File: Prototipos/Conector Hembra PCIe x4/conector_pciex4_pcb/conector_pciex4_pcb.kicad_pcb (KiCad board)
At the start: 2 copper layers, 16.4 x 39.7 mm, 33 parts, among them J1 10018783-10211TLF

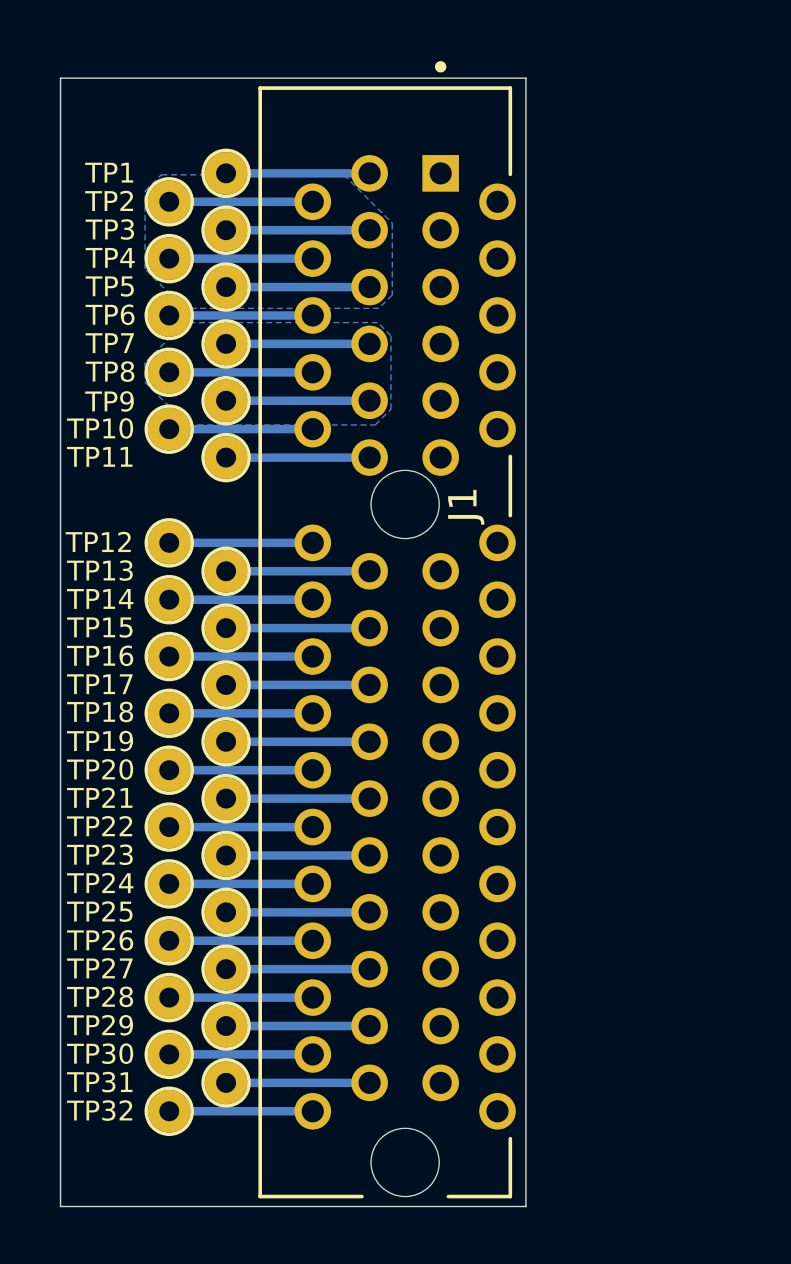
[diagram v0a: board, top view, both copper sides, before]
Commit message: Corrección PCB
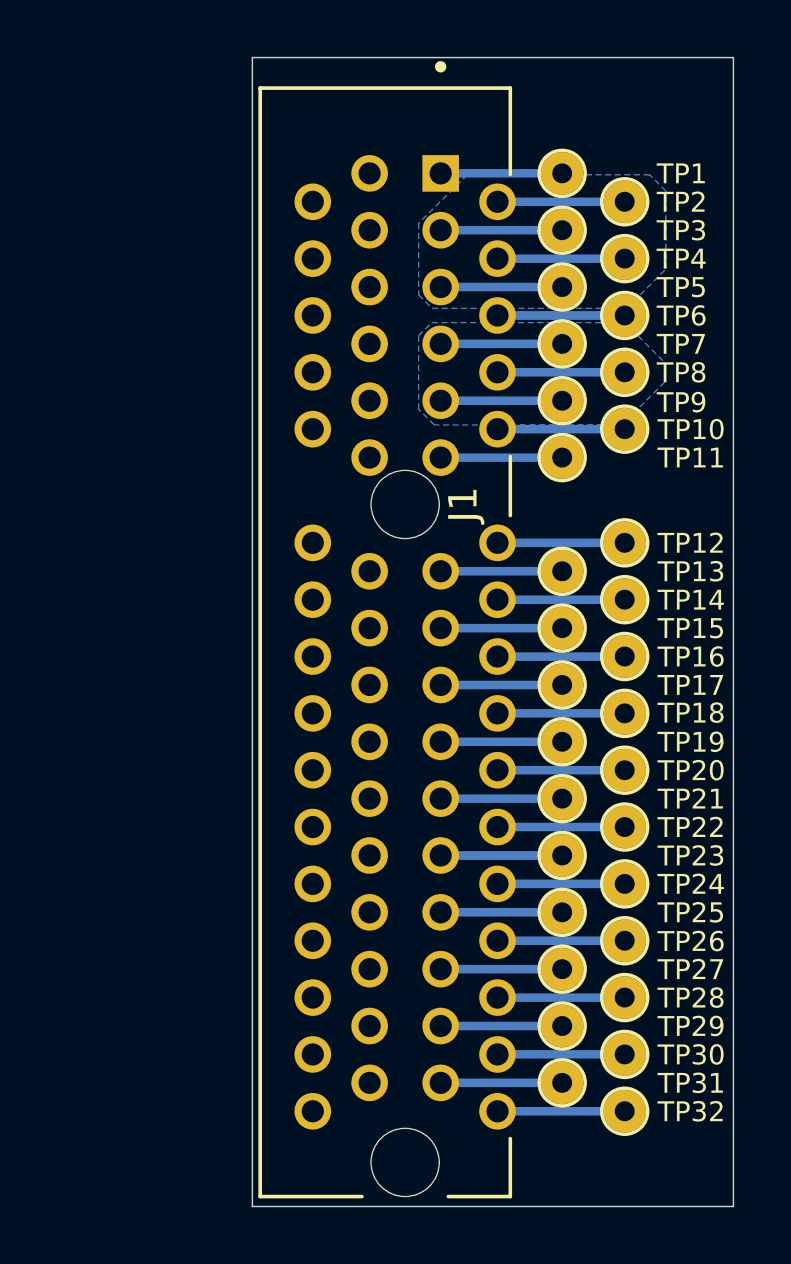
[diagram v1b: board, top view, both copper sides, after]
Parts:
- moved TP10 16.0 mm to (140.4, 73.6)
- moved TP12 16.0 mm to (140.4, 77.6)
- moved TP14 16.0 mm to (140.4, 79.6)
- moved TP16 16.0 mm to (140.4, 81.6)
- moved TP18 16.0 mm to (140.4, 83.6)
- moved TP2 16.0 mm to (140.4, 65.6)
- moved TP20 16.0 mm to (140.4, 85.6)
- moved TP22 16.0 mm to (140.4, 87.6)
- moved TP24 16.0 mm to (140.4, 89.6)
- moved TP26 16.0 mm to (140.4, 91.6)
- moved TP28 16.0 mm to (140.4, 93.6)
- moved TP30 16.0 mm to (140.4, 95.6)
- moved TP32 16.0 mm to (140.4, 97.6)
- moved TP4 16.0 mm to (140.4, 67.6)
- moved TP6 16.0 mm to (140.4, 69.6)
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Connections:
- J1 pad A1: unconnected-(J1-PadA1) -> Net-(J1-PadA1)
- J1 pad A10: unconnected-(J1-PadA10) -> Net-(J1-PadA10)
- J1 pad A11: unconnected-(J1-PadA11) -> Net-(J1-PadA11)
- J1 pad A12: unconnected-(J1-PadA12) -> Net-(J1-PadA12)
- J1 pad A13: unconnected-(J1-PadA13) -> Net-(J1-PadA13)
- J1 pad A14: unconnected-(J1-PadA14) -> Net-(J1-PadA14)
- J1 pad A15: unconnected-(J1-PadA15) -> Net-(J1-PadA15)
- J1 pad A16: unconnected-(J1-PadA16) -> Net-(J1-PadA16)
- J1 pad A17: unconnected-(J1-PadA17) -> Net-(J1-PadA17)
- J1 pad A18: unconnected-(J1-PadA18) -> Net-(J1-PadA18)
- J1 pad A19: unconnected-(J1-PadA19) -> Net-(J1-PadA19)
- J1 pad A2: unconnected-(J1-PadA2) -> Net-(J1-PadA2)
- J1 pad A20: unconnected-(J1-PadA20) -> Net-(J1-PadA20)
- J1 pad A21: unconnected-(J1-PadA21) -> Net-(J1-PadA21)
- J1 pad A22: unconnected-(J1-PadA22) -> Net-(J1-PadA22)
- J1 pad A23: unconnected-(J1-PadA23) -> Net-(J1-PadA23)
- J1 pad A24: unconnected-(J1-PadA24) -> Net-(J1-PadA24)
- J1 pad A25: unconnected-(J1-PadA25) -> Net-(J1-PadA25)
- J1 pad A26: unconnected-(J1-PadA26) -> Net-(J1-PadA26)
- J1 pad A27: unconnected-(J1-PadA27) -> Net-(J1-PadA27)
- J1 pad A28: unconnected-(J1-PadA28) -> Net-(J1-PadA28)
- J1 pad A29: unconnected-(J1-PadA29) -> Net-(J1-PadA29)
- J1 pad A3: unconnected-(J1-PadA3) -> Net-(J1-PadA2)
- J1 pad A30: unconnected-(J1-PadA30) -> Net-(J1-PadA30)
- J1 pad A31: unconnected-(J1-PadA31) -> Net-(J1-PadA31)
- J1 pad A32: unconnected-(J1-PadA32) -> Net-(J1-PadA32)
- J1 pad A4: unconnected-(J1-PadA4) -> Net-(J1-PadA2)
- J1 pad A5: unconnected-(J1-PadA5) -> Net-(J1-PadA2)
- J1 pad A6: unconnected-(J1-PadA6) -> Net-(J1-PadA6)
- J1 pad A7: unconnected-(J1-PadA7) -> Net-(J1-PadA7)
- J1 pad A8: unconnected-(J1-PadA8) -> Net-(J1-PadA7)
- J1 pad A9: unconnected-(J1-PadA9) -> Net-(J1-PadA7)
- J1 pad B1: Net-(J1-PadB1) -> unconnected-(J1-PadB1)
- J1 pad B10: Net-(J1-PadB10) -> unconnected-(J1-PadB10)
- J1 pad B11: Net-(J1-PadB11) -> unconnected-(J1-PadB11)
- J1 pad B12: Net-(J1-PadB12) -> unconnected-(J1-PadB12)
- J1 pad B13: Net-(J1-PadB13) -> unconnected-(J1-PadB13)
- J1 pad B14: Net-(J1-PadB14) -> unconnected-(J1-PadB14)
- J1 pad B15: Net-(J1-PadB15) -> unconnected-(J1-PadB15)
- J1 pad B16: Net-(J1-PadB16) -> unconnected-(J1-PadB16)
- J1 pad B17: Net-(J1-PadB17) -> unconnected-(J1-PadB17)
- J1 pad B18: Net-(J1-PadB18) -> unconnected-(J1-PadB18)
- J1 pad B19: Net-(J1-PadB19) -> unconnected-(J1-PadB19)
- J1 pad B2: Net-(J1-PadB2) -> unconnected-(J1-PadB2)
- J1 pad B20: Net-(J1-PadB20) -> unconnected-(J1-PadB20)
- J1 pad B21: Net-(J1-PadB21) -> unconnected-(J1-PadB21)
- J1 pad B22: Net-(J1-PadB22) -> unconnected-(J1-PadB22)
- J1 pad B23: Net-(J1-PadB23) -> unconnected-(J1-PadB23)
- J1 pad B24: Net-(J1-PadB24) -> unconnected-(J1-PadB24)
- J1 pad B25: Net-(J1-PadB25) -> unconnected-(J1-PadB25)
- J1 pad B26: Net-(J1-PadB26) -> unconnected-(J1-PadB26)
- J1 pad B27: Net-(J1-PadB27) -> unconnected-(J1-PadB27)
- J1 pad B28: Net-(J1-PadB28) -> unconnected-(J1-PadB28)
- J1 pad B29: Net-(J1-PadB29) -> unconnected-(J1-PadB29)
- J1 pad B3: Net-(J1-PadB2) -> unconnected-(J1-PadB3)
- J1 pad B30: Net-(J1-PadB30) -> unconnected-(J1-PadB30)
- J1 pad B31: Net-(J1-PadB31) -> unconnected-(J1-PadB31)
- J1 pad B32: Net-(J1-PadB32) -> unconnected-(J1-PadB32)
- J1 pad B4: Net-(J1-PadB2) -> unconnected-(J1-PadB4)
- J1 pad B5: Net-(J1-PadB2) -> unconnected-(J1-PadB5)
- J1 pad B6: Net-(J1-PadB6) -> unconnected-(J1-PadB6)
- J1 pad B7: Net-(J1-PadB7) -> unconnected-(J1-PadB7)
- J1 pad B8: Net-(J1-PadB7) -> unconnected-(J1-PadB8)
- J1 pad B9: Net-(J1-PadB7) -> unconnected-(J1-PadB9)
- TP1 pad 1: Net-(J1-PadB1) -> Net-(J1-PadA1)
- TP10 pad 1: Net-(J1-PadB10) -> Net-(J1-PadA10)
- TP11 pad 1: Net-(J1-PadB11) -> Net-(J1-PadA11)
- TP12 pad 1: Net-(J1-PadB12) -> Net-(J1-PadA12)
- TP13 pad 1: Net-(J1-PadB13) -> Net-(J1-PadA13)
- TP14 pad 1: Net-(J1-PadB14) -> Net-(J1-PadA14)
- TP15 pad 1: Net-(J1-PadB15) -> Net-(J1-PadA15)
- TP16 pad 1: Net-(J1-PadB16) -> Net-(J1-PadA16)
- TP17 pad 1: Net-(J1-PadB17) -> Net-(J1-PadA17)
- TP18 pad 1: Net-(J1-PadB18) -> Net-(J1-PadA18)
- TP19 pad 1: Net-(J1-PadB19) -> Net-(J1-PadA19)
- TP2 pad 1: Net-(J1-PadB2) -> Net-(J1-PadA2)
- TP20 pad 1: Net-(J1-PadB20) -> Net-(J1-PadA20)
- TP21 pad 1: Net-(J1-PadB21) -> Net-(J1-PadA21)
- TP22 pad 1: Net-(J1-PadB22) -> Net-(J1-PadA22)
- TP23 pad 1: Net-(J1-PadB23) -> Net-(J1-PadA23)
- TP24 pad 1: Net-(J1-PadB24) -> Net-(J1-PadA24)
- TP25 pad 1: Net-(J1-PadB25) -> Net-(J1-PadA25)
- TP26 pad 1: Net-(J1-PadB26) -> Net-(J1-PadA26)
- TP27 pad 1: Net-(J1-PadB27) -> Net-(J1-PadA27)
- TP28 pad 1: Net-(J1-PadB28) -> Net-(J1-PadA28)
- TP29 pad 1: Net-(J1-PadB29) -> Net-(J1-PadA29)
- TP3 pad 1: Net-(J1-PadB2) -> Net-(J1-PadA2)
- TP30 pad 1: Net-(J1-PadB30) -> Net-(J1-PadA30)
- TP31 pad 1: Net-(J1-PadB31) -> Net-(J1-PadA31)
- TP32 pad 1: Net-(J1-PadB32) -> Net-(J1-PadA32)
- TP4 pad 1: Net-(J1-PadB2) -> Net-(J1-PadA2)
- TP5 pad 1: Net-(J1-PadB2) -> Net-(J1-PadA2)
- TP6 pad 1: Net-(J1-PadB6) -> Net-(J1-PadA6)
- TP7 pad 1: Net-(J1-PadB7) -> Net-(J1-PadA7)
- TP8 pad 1: Net-(J1-PadB7) -> Net-(J1-PadA7)
- TP9 pad 1: Net-(J1-PadB7) -> Net-(J1-PadA7)
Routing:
- net Net-(J1-PadB2): track 20.2 -> 0.00 mm
- net Net-(J1-PadA2): track 0.00 -> 17.5 mm
- net Net-(J1-PadB7): track 15.2 -> 0.00 mm
- net Net-(J1-PadA7): track 0.00 -> 13.0 mm
- net Net-(J1-PadB6): track 5.05 -> 0.00 mm
- net Net-(J1-PadB32): track 5.05 -> 0.00 mm
- net Net-(J1-PadB31): track 5.05 -> 0.00 mm
- net Net-(J1-PadB30): track 5.05 -> 0.00 mm
- net Net-(J1-PadB29): track 5.05 -> 0.00 mm
- net Net-(J1-PadB28): track 5.05 -> 0.00 mm
- net Net-(J1-PadB27): track 5.05 -> 0.00 mm
- net Net-(J1-PadB26): track 5.05 -> 0.00 mm
- net Net-(J1-PadB25): track 5.05 -> 0.00 mm
- net Net-(J1-PadB24): track 5.05 -> 0.00 mm
- net Net-(J1-PadB23): track 5.05 -> 0.00 mm
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- added copper zone on B.Cu, net Net-(J1-PadA2)
- added copper zone on B.Cu, net Net-(J1-PadA7)
- removed copper zone on B.Cu, net Net-(J1-PadB2)
- removed copper zone on B.Cu, net Net-(J1-PadB7)
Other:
- board size 16.4 x 39.7 mm -> 16.9 x 40.4 mm
